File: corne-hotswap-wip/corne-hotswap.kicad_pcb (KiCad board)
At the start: 2 copper layers, 133.8 x 91.7 mm, 49 parts, among them J1 Battery Connector, J2 nice!view, J3 USB_C_Receptacle_PowerOnly_6P, J4 Battery Wire, SW1 SW_Push, SW10 SW_Push, SW11 SW_Push, SW12 SW_Push, SW13 SW_Push, SW14 SW_Push, SW15 SW_Push, SW16 SW_Push, SW17 SW_Push, SW18 SW_Push, SW19 SW_Push, SW2 SW_Push, SW20 SW_Push, SW21 SW_Push, SW3 SW_Push, SW4 SW_Push, SW5 SW_Push, SW6 SW_Push, SW7 SW_Push, SW8 SW_Push, SW9 SW_Push, U1 ProMicro

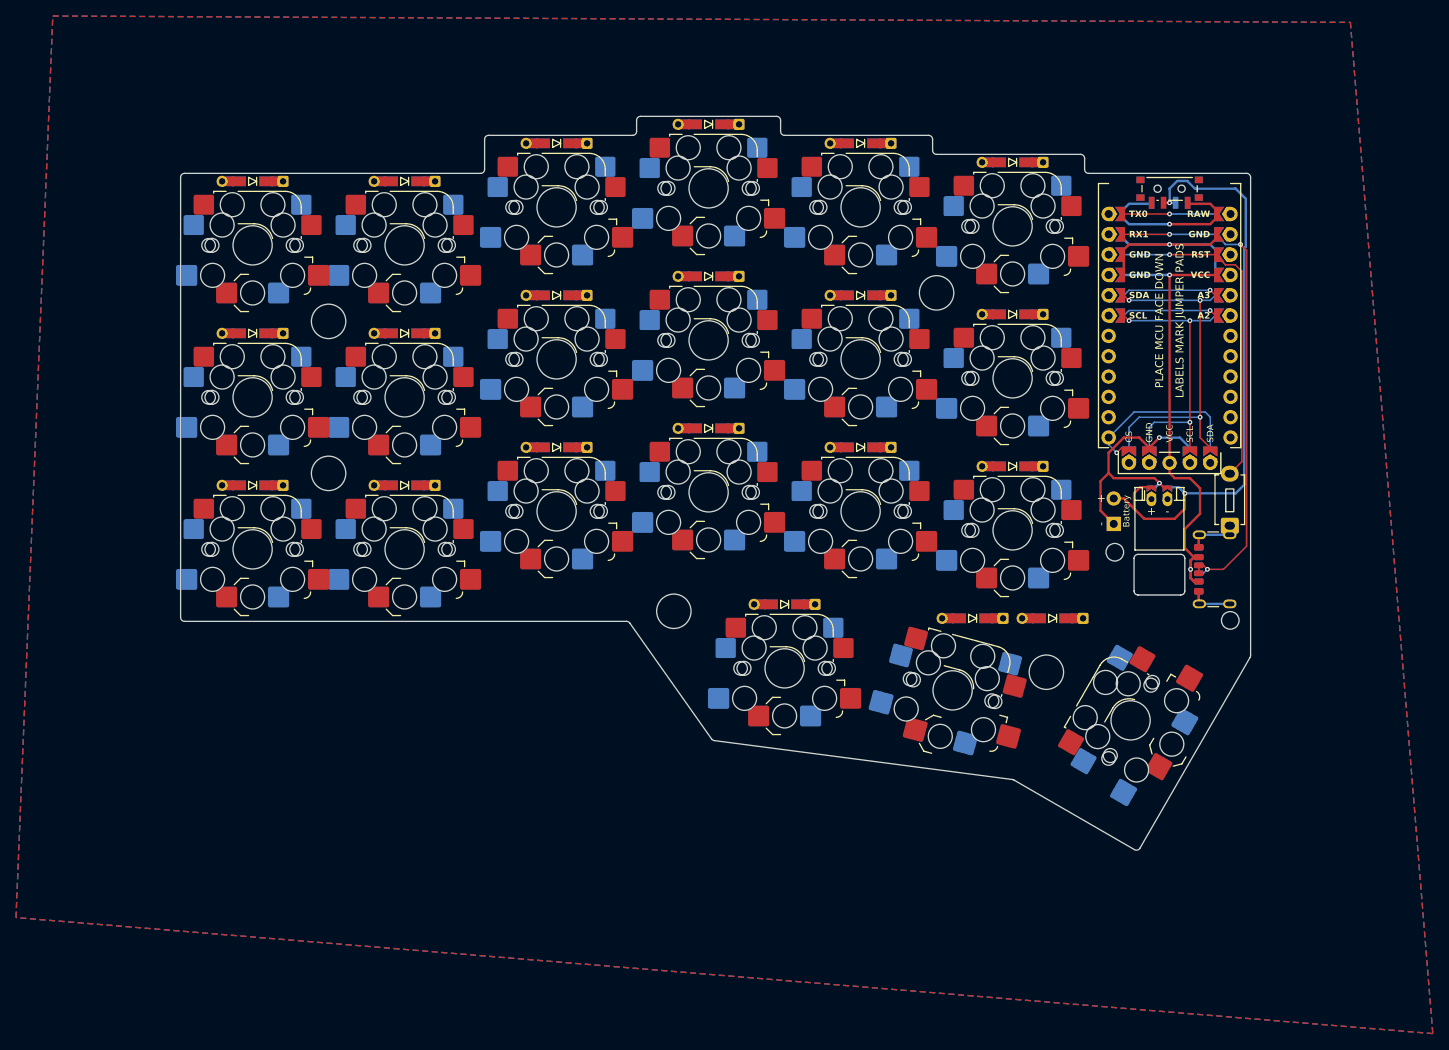
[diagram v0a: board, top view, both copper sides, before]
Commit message: column wiring
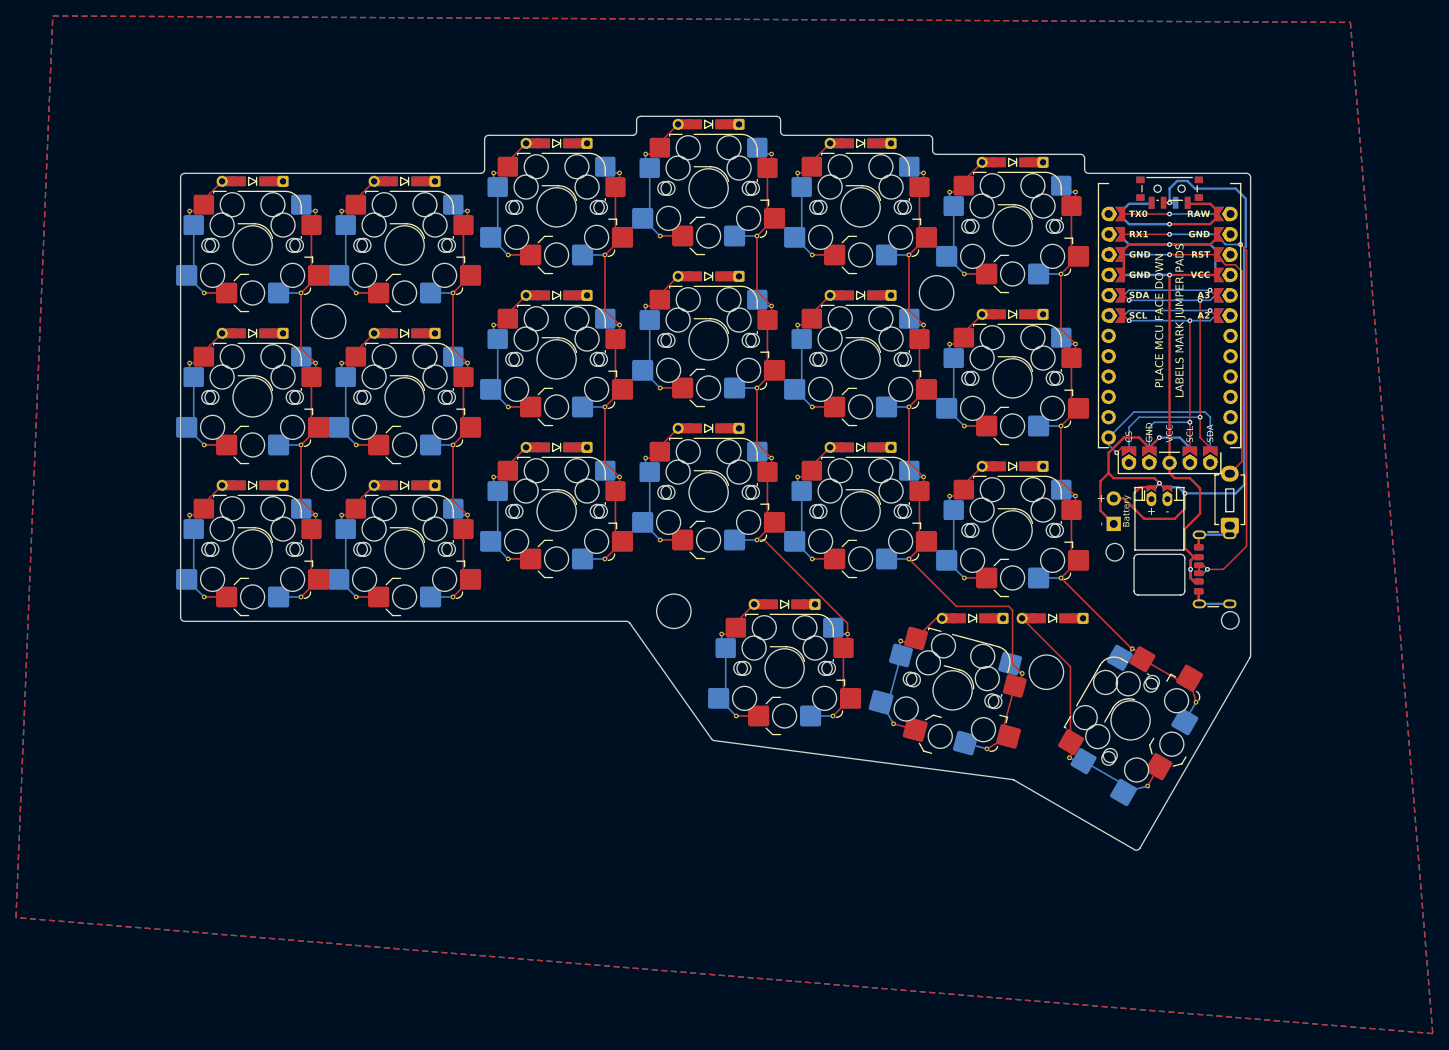
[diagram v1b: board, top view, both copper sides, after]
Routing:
- net col4: track 0.00 -> 43.0 mm
- net col3: track 0.00 -> 36.0 mm
- net col5: track 0.00 -> 31.6 mm
- net col0: track 12.0 -> 31.0 mm
- net col2: track 0.00 -> 19.0 mm
- net col1: track 12.0 -> 31.0 mm
- net Net-(D21-A): track 0.00 -> 18.0 mm
- net Net-(D17-A): track 0.00 -> 4.30 mm
- net Net-(D9-A): track 0.00 -> 3.86 mm
- net Net-(D8-A): track 0.00 -> 3.86 mm
- net Net-(D7-A): track 0.00 -> 3.86 mm
- net Net-(D6-A): track 0.00 -> 3.86 mm
- net Net-(D5-A): track 0.00 -> 3.86 mm
- net Net-(D4-A): track 0.00 -> 3.86 mm
- net Net-(D3-A): track 0.00 -> 3.86 mm
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
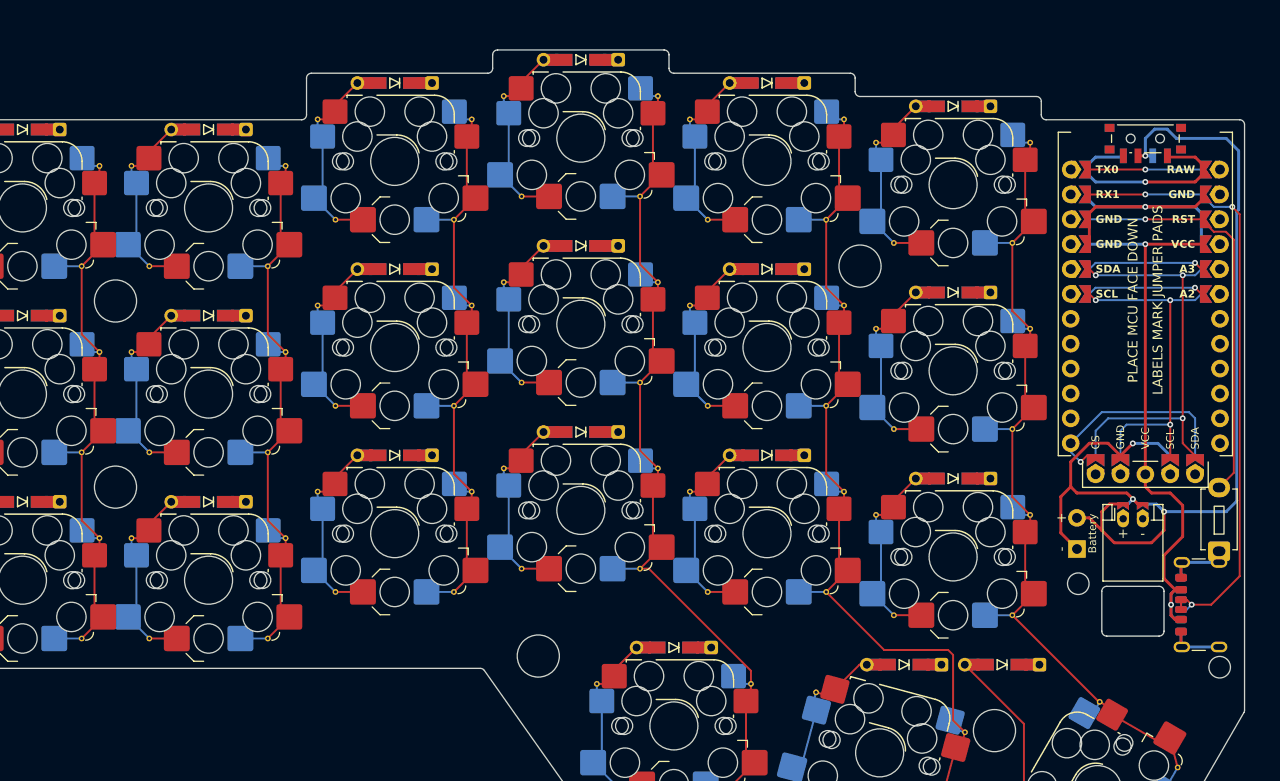
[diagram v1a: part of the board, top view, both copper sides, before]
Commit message: wiring
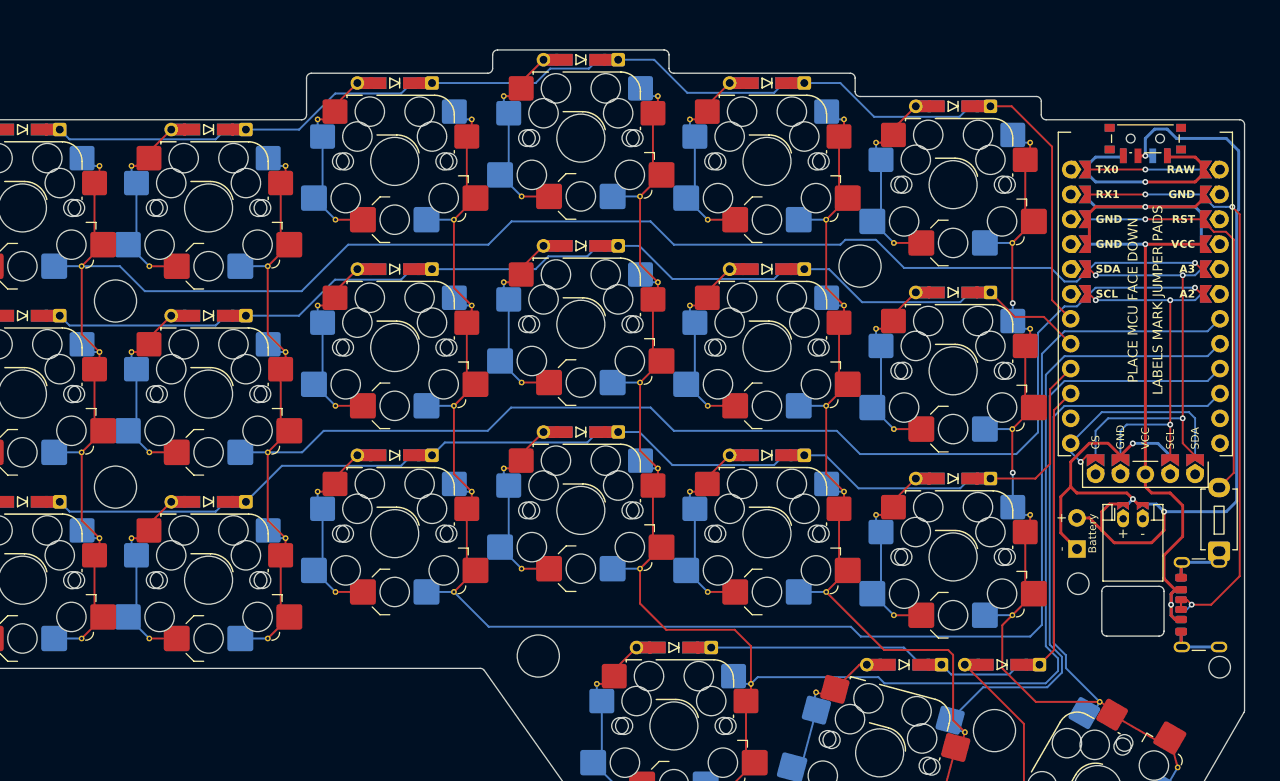
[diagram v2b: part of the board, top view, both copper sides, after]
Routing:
- net row0: track 0.00 -> 119.3 mm
- net col0: track 31.0 -> 141.3 mm
- net col2: track 19.0 -> 128.8 mm
- net row2: track 0.00 -> 109.3 mm
- net row1: track 0.00 -> 102.3 mm
- net col1: track 31.0 -> 131.4 mm
- net col3: track 36.0 -> 121.8 mm
- net col4: track 43.0 -> 103.8 mm
- net row3: track 0.00 -> 59.9 mm
- net col5: track 31.6 -> 82.2 mm, vias 0 -> 2
